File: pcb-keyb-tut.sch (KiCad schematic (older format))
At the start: 24 parts, among them SW1 SW_Push, U1 ATmega32U4-AU, Y1 16MHz

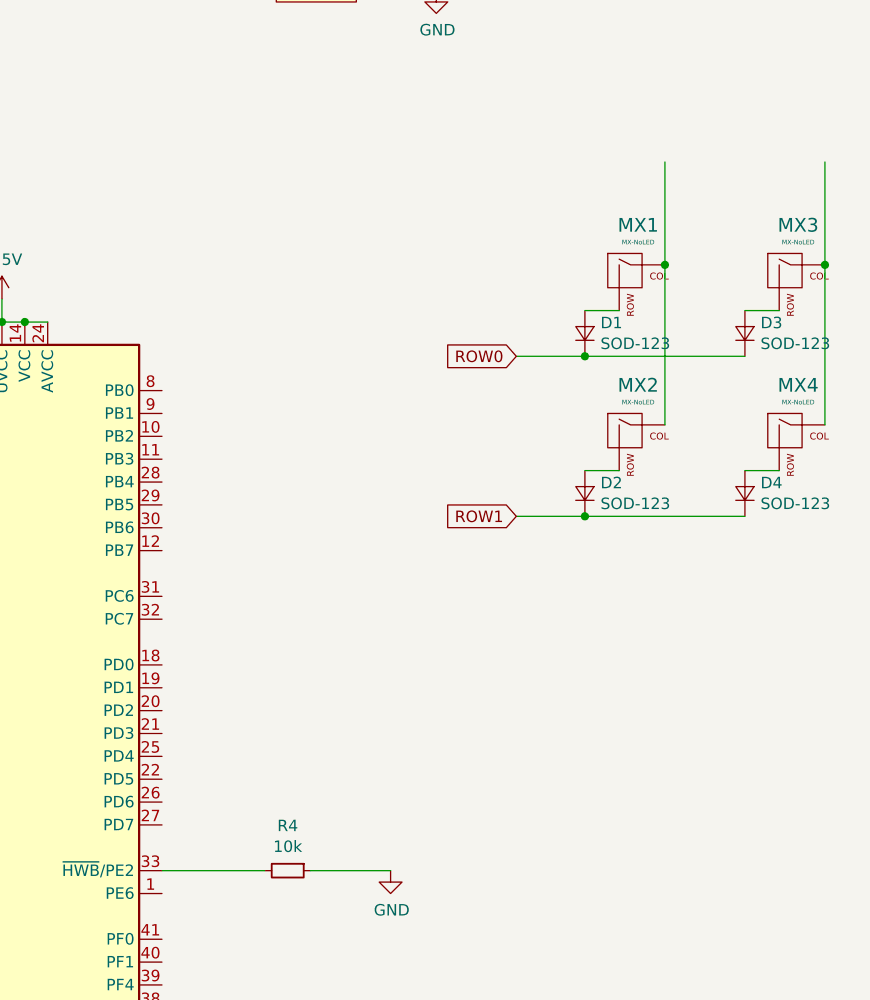
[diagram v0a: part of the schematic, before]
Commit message: DONE
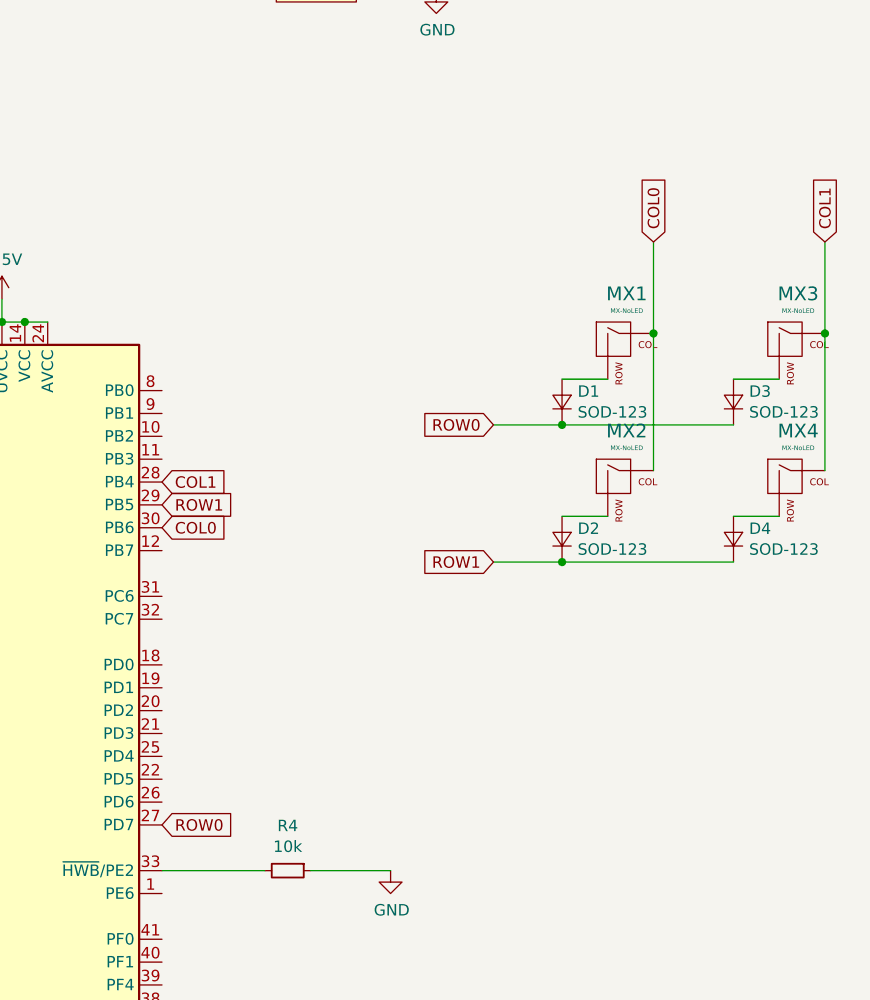
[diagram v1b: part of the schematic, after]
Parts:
- MX1, MX2, MX3, MX4: footprint (none) -> MX_Alps_Hybrid:MX-1U
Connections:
- net labels added: COL0, COL1
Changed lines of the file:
@@
 EESchema Schematic File Version 4
+LIBS:pcb-keyb-tut-cache
 EELAYER 30 0
 EELAYER END
@@
 $Comp
 L MX_Alps_Hybrid:MX-NoLED MX1
-U 1 1 6294733C
-P 6500 3150
-F 0 "MX1" H 6533 3373 60  0000 C CNN
-F 1 "MX-NoLED" H 6533 3299 20  0000 C CNN
-F 2 "" H 5875 3125 60  0001 C CNN
-F 3 "" H 5875 3125 60  0001 C CNN
-	1    6500 3150
+U 1 1 628D5AD1
+P 6450 3450
+F 0 "MX1" H 6483 3673 60  0000 C CNN
+F 1 "MX-NoLED" H 6483 3599 20  0000 C CNN
+F 2 "MX_Alps_Hybrid:MX-1U" H 5825 3425 60  0001 C CNN
+F 3 "" H 5825 3425 60  0001 C CNN
+	1    6450 3450
+	1    0    0    -1
+$EndComp
+$Comp
+L MX_Alps_Hybrid:MX-NoLED MX3
+U 1 1 628DC010
+P 7200 3450
+F 0 "MX3" H 7233 3673 60  0000 C CNN
+F 1 "MX-NoLED" H 7233 3599 20  0000 C CNN
+F 2 "MX_Alps_Hybrid:MX-1U" H 6575 3425 60  0001 C CNN
+F 3 "" H 6575 3425 60  0001 C CNN
+	1    7200 3450
+	1    0    0    -1
+$EndComp
+$Comp
+L MX_Alps_Hybrid:MX-NoLED MX2
+U 1 1 628DCF00
+P 6450 4050
+F 0 "MX2" H 6483 4273 60  0000 C CNN
+F 1 "MX-NoLED" H 6483 4199 20  0000 C CNN
+F 2 "MX_Alps_Hybrid:MX-1U" H 5825 4025 60  0001 C CNN
+F 3 "" H 5825 4025 60  0001 C CNN
+	1    6450 4050
+	1    0    0    -1
+$EndComp
+$Comp
+L MX_Alps_Hybrid:MX-NoLED MX4
+U 1 1 628DE09D
+P 7200 4050
+F 0 "MX4" H 7233 4273 60  0000 C CNN
+F 1 "MX-NoLED" H 7233 4199 20  0000 C CNN
+F 2 "MX_Alps_Hybrid:MX-1U" H 6575 4025 60  0001 C CNN
+F 3 "" H 6575 4025 60  0001 C CNN
+	1    7200 4050
 	1    0    0    -1
 $EndComp
 $Comp
 L Device:D_Small D1
-U 1 1 62947FDB
-P 6300 3400
-F 0 "D1" V 6346 3332 50  0000 R CNN
-F 1 "SOD-123" V 6255 3332 50  0000 R CNN
-F 2 "Diode_SMD:D_SOD-123" V 6300 3400 50  0001 C CNN
-F 3 "~" V 6300 3400 50  0001 C CNN
-	1    6300 3400
+U 1 1 628E1F00
+P 6200 3700
+F 0 "D1" V 6246 3632 50  0000 R CNN
+F 1 "SOD-123" V 6155 3632 50  0000 R CNN
+F 2 "Diode_SMD:D_SOD-123" V 6200 3700 50  0001 C CNN
+F 3 "~" V 6200 3700 50  0001 C CNN
+	1    6200 3700
 	0    -1   -1   0
 $EndComp
-Wire Wire Line
-	6450 3300 6300 3300
-$Comp
-L MX_Alps_Hybrid:MX-NoLED MX3
-U 1 1 6294B3F0
-P 7200 3150
-F 0 "MX3" H 7233 3373 60  0000 C CNN
-F 1 "MX-NoLED" H 7233 3299 20  0000 C CNN
-F 2 "" H 6575 3125 60  0001 C CNN
-F 3 "" H 6575 3125 60  0001 C CNN
-	1    7200 3150
-	1    0    0    -1
-$EndComp
 $Comp
 L Device:D_Small D3
-U 1 1 6294B3FA
-P 7000 3400
-F 0 "D3" V 7046 3332 50  0000 R CNN
-F 1 "SOD-123" V 6955 3332 50  0000 R CNN
-F 2 "Diode_SMD:D_SOD-123" V 7000 3400 50  0001 C CNN
-F 3 "~" V 7000 3400 50  0001 C CNN
-	1    7000 3400
+U 1 1 628E59C2
+P 6950 3700
+F 0 "D3" V 6996 3632 50  0000 R CNN
+F 1 "SOD-123" V 6905 3632 50  0000 R CNN
+F 2 "Diode_SMD:D_SOD-123" V 6950 3700 50  0001 C CNN
+F 3 "~" V 6950 3700 50  0001 C CNN
+	1    6950 3700
 	0    -1   -1   0
 $EndComp
-Wire Wire Line
-	7150 3300 7000 3300
-$Comp
-L MX_Alps_Hybrid:MX-NoLED MX2
-U 1 1 6294DD5C
-P 6500 3850
-F 0 "MX2" H 6533 4073 60  0000 C CNN
-F 1 "MX-NoLED" H 6533 3999 20  0000 C CNN
-F 2 "" H 5875 3825 60  0001 C CNN
-F 3 "" H 5875 3825 60  0001 C CNN
-	1    6500 3850
-	1    0    0    -1
+$Comp
+L Device:D_Small D4
+U 1 1 628E7A19
+P 6950 4300
+F 0 "D4" V 6996 4232 50  0000 R CNN
+F 1 "SOD-123" V 6905 4232 50  0000 R CNN
+F 2 "Diode_SMD:D_SOD-123" V 6950 4300 50  0001 C CNN
+F 3 "~" V 6950 4300 50  0001 C CNN
+	1    6950 4300
+	0    -1   -1   0
 $EndComp
 $Comp
 L Device:D_Small D2
-U 1 1 6294DD66
-P 6300 4100
-F 0 "D2" V 6346 4032 50  0000 R CNN
-F 1 "SOD-123" V 6255 4032 50  0000 R CNN
-F 2 "Diode_SMD:D_SOD-123" V 6300 4100 50  0001 C CNN
-F 3 "~" V 6300 4100 50  0001 C CNN
-	1    6300 4100
+U 1 1 628ECE80
+P 6200 4300
+F 0 "D2" V 6246 4232 50  0000 R CNN
+F 1 "SOD-123" V 6155 4232 50  0000 R CNN
+F 2 "Diode_SMD:D_SOD-123" V 6200 4300 50  0001 C CNN
+F 3 "~" V 6200 4300 50  0001 C CNN
+	1    6200 4300
 	0    -1   -1   0
 $EndComp
 Wire Wire Line
-	6450 4000 6300 4000
-$Comp
-L MX_Alps_Hybrid:MX-NoLED MX4
-U 1 1 62950EDC
-P 7200 3850
-F 0 "MX4" H 7233 4073 60  0000 C CNN
-F 1 "MX-NoLED" H 7233 3999 20  0000 C CNN
-F 2 "" H 6575 3825 60  0001 C CNN
-F 3 "" H 6575 3825 60  0001 C CNN
-	1    7200 3850
-	1    0    0    -1
-$EndComp
-$Comp
-L Device:D_Small D4
-U 1 1 62950EE6
-P 7000 4100
-F 0 "D4" V 7046 4032 50  0000 R CNN
-F 1 "SOD-123" V 6955 4032 50  0000 R CNN
-F 2 "Diode_SMD:D_SOD-123" V 7000 4100 50  0001 C CNN
-F 3 "~" V 7000 4100 50  0001 C CNN
-	1    7000 4100
-	0    -1   -1   0
-$EndComp
-Wire Wire Line
-	7150 4000 7000 4000
-Wire Wire Line
-	6650 3100 6650 3800
-Wire Wire Line
-	6300 3500 7000 3500
-Wire Wire Line
-	6300 3500 6000 3500
-Connection ~ 6300 3500
-Wire Wire Line
-	6300 4200 6000 4200
-Connection ~ 6300 4200
-Wire Wire Line
-	6300 4200 7000 4200
-Wire Wire Line
-	7350 3800 7350 3100
-Connection ~ 7350 3100
-Wire Wire Line
-	7350 3100 7350 2650
-Wire Wire Line
-	6650 3100 6650 2650
-Connection ~ 6650 3100
-Text GLabel 6000 3500 0    50   Input ~ 0
+	6400 4200 6200 4200
+Wire Wire Line
+	7150 4200 6950 4200
+Wire Wire Line
+	7150 3600 6950 3600
+Wire Wire Line
+	6400 3600 6200 3600
+Wire Wire Line
+	6600 4000 6600 3400
+Connection ~ 6600 3400
+Wire Wire Line
+	6600 3400 6600 3000
+Wire Wire Line
+	7350 4000 7350 3400
+Connection ~ 7350 3400
+Wire Wire Line
+	7350 3400 7350 3000
+Wire Wire Line
+	6950 3800 6200 3800
+Connection ~ 6200 3800
+Wire Wire Line
+	6200 3800 5900 3800
+Wire Wire Line
+	6950 4400 6200 4400
+Connection ~ 6200 4400
+Wire Wire Line
+	6200 4400 5900 4400
+Text GLabel 5900 3800 0    50   Input ~ 0
 ROW0
-Text GLabel 6000 4200 0    50   Input ~ 0
+Text GLabel 5900 4400 0    50   Input ~ 0
+ROW1
+Text GLabel 6600 3000 1    50   Input ~ 0
+COL0
+Text GLabel 7350 3000 1    50   Input ~ 0
+COL1
+Text GLabel 4450 4250 2    50   Input ~ 0
+COL0
+Text GLabel 4450 5550 2    50   Input ~ 0
+ROW0
+Text GLabel 4450 4050 2    50   Input ~ 0
+COL1
+Text GLabel 4450 4150 2    50   Input ~ 0
 ROW1
 $EndSCHEMATC
